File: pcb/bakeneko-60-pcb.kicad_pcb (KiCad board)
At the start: 2 copper layers, 284.7 x 94.2 mm, 154 parts, among them J1 JST SH 4-pin, J2 AVR-ISP-6, SW1 Reset, U1 SRV05-4, U2 ATmega32U4-AU, Y1 16MHz

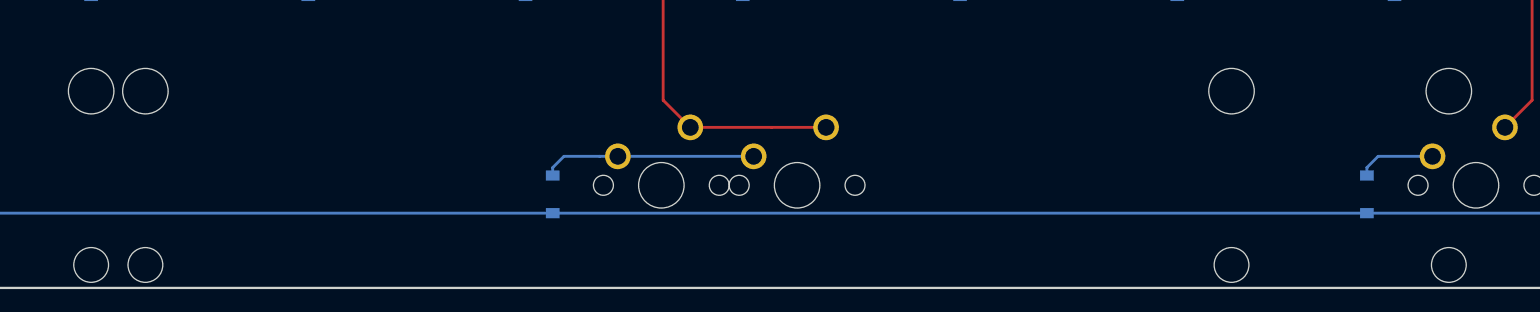
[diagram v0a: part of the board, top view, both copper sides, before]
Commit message: Remove spacebars
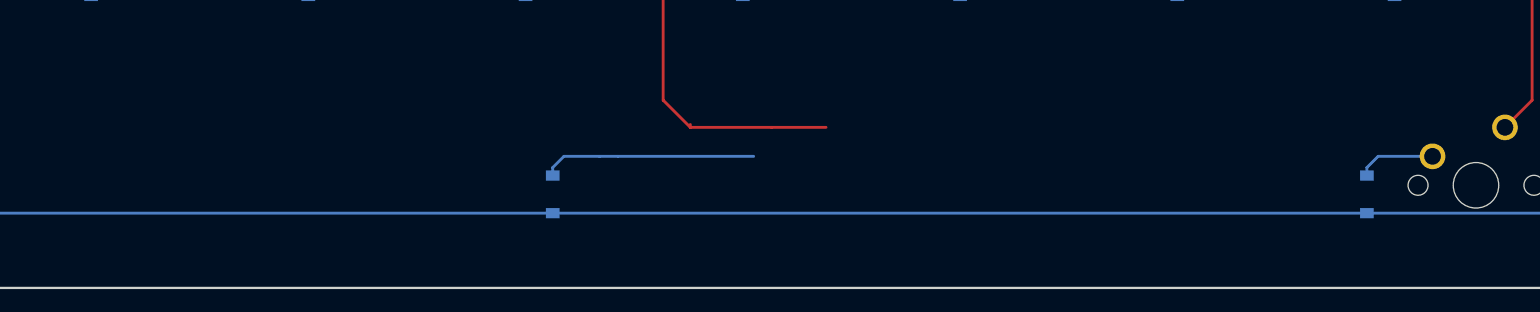
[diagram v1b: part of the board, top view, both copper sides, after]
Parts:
- removed the MX62 at (130.4, 85.2)
- removed MX70: 7u, MX_Only:MXOnly-7U-ReversedStabilizers-NoLED
- renumbered MX63 to MX62, MX64 to MX63, MX65 to MX64, MX66 to MX65, MX67 to MX66, MX68 to MX67, MX69 to MX68, MX72 to MX71, MX73 to MX72
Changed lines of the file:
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@@
     (at 201.88125 85.2)
     (attr through_hole)
-    (fp_text reference "MX63" (at 0 3.175) (layer "Dwgs.User")
+    (fp_text reference "MX62" (at 0 3.175) (layer "Dwgs.User")
       (effects (font (size 1 1) (thickness 0.15)))
     )
@@
     (at 225.69375 85.2)
     (attr through_hole)
-    (fp_text reference "MX64" (at 0 3.175) (layer "Dwgs.User")
+    (fp_text reference "MX63" (at 0 3.175) (layer "Dwgs.User")
       (effects (font (size 1 1) (thickness 0.15)))
     )
@@
     (at 249.50625 85.2)
     (attr through_hole)
-    (fp_text reference "MX65" (at 0 3.175) (layer "Dwgs.User")
+    (fp_text reference "MX64" (at 0 3.175) (layer "Dwgs.User")
       (effects (font (size 1 1) (thickness 0.15)))
     )
@@
     (at 273.31875 85.2)
     (attr through_hole)
-    (fp_text reference "MX66" (at 0 3.175) (layer "Dwgs.User")
+    (fp_text reference "MX65" (at 0 3.175) (layer "Dwgs.User")
       (effects (font (size 1 1) (thickness 0.15)))
     )
@@
     (at 37.575 85.2)
     (attr through_hole)
-    (fp_text reference "MX68" (at 0 3.175) (layer "Dwgs.User")
+    (fp_text reference "MX67" (at 0 3.175) (layer "Dwgs.User")
       (effects (font (size 1 1) (thickness 0.15)))
     )
@@
     (at 61.3875 85.2)
     (attr through_hole)
-    (fp_text reference "MX69" (at 0 3.175) (layer "Dwgs.User")
+    (fp_text reference "MX68" (at 0 3.175) (layer "Dwgs.User")
       (effects (font (size 1 1) (thickness 0.15)))
     )
@@
       (net 80 "COL2"))
   )
-  (footprint "MX_Only:MXOnly-7U-ReversedStabilizers-NoLED" (layer "F.Cu")
-    (at 142.35 85.2)
-    (attr through_hole)
-    (fp_text reference "MX70" (at 0 3.175) (layer "Dwgs.User")
-      (effects (font (size 1 1) (thickness 0.15)))
-    )
-    (fp_text value "7u" (at 0 -7.9375) (layer "Dwgs.User")
-      (effects (font (size 1 1) (thickness 0.15)))
-    )
-    (fp_line (start -7 7) (end -5 7) (layer "Dwgs.User") (width 0.15))
-    (fp_line (start -5 -7) (end -7 -7) (layer "Dwgs.User") (width 0.15))
-    (fp_line (start 5 -7) (end 7 -7) (layer "Dwgs.User") (width 0.15))
-    (fp_line (start -7 5) (end -7 7) (layer "Dwgs.User") (width 0.15))
-    (fp_line (start 7 -7) (end 7 -5) (layer "Dwgs.User") (width 0.15))
-    (fp_line (start 5 7) (end 7 7) (layer "Dwgs.User") (width 0.15))
-    (fp_line (start -7 -7) (end -7 -5) (layer "Dwgs.User") (width 0.15))
-    (fp_line (start 7 7) (end 7 5) (layer "Dwgs.User") (width 0.15))
-    (fp_line (start -66.675 -9.525) (end 66.675 -9.525) (layer "Dwgs.User") (width 0.15))
-    (fp_line (start 66.675 -9.525) (end 66.675 9.525) (layer "Dwgs.User") (width 0.15))
-    (fp_line (start -66.675 9.525) (end -66.675 -9.525) (layer "Dwgs.User") (width 0.15))
-    (fp_line (start -66.675 9.525) (end 66.675 9.525) (layer "Dwgs.User") (width 0.15))
-    (pad "" np_thru_hole circle locked (at -57.15 -8.255) (size 3.9878 3.9878) (drill 3.9878) (layers *.Cu *.Mask))
-    (pad "" np_thru_hole circle locked (at 0 0) (size 3.9878 3.9878) (drill 3.9878) (layers *.Cu *.Mask))
-    (pad "" np_thru_hole circle locked (at 57.15 -8.255) (size 3.9878 3.9878) (drill 3.9878) (layers *.Cu *.Mask))
-    (pad "" np_thru_hole circle locked (at -57.15 6.985) (size 3.048 3.048) (drill 3.048) (layers *.Cu *.Mask))
-    (pad "" np_thru_hole circle locked (at 5.08 0 48.0996) (size 1.75 1.75) (drill 1.75) (layers *.Cu *.Mask))
-    (pad "" np_thru_hole circle locked (at -5.08 0 48.0996) (size 1.75 1.75) (drill 1.75) (layers *.Cu *.Mask))
-    (pad "" np_thru_hole circle locked (at 57.15 6.985) (size 3.048 3.048) (drill 3.048) (layers *.Cu *.Mask))
-    (pad "1" thru_hole circle locked (at -3.81 -2.54) (size 2.25 2.25) (drill 1.47) (layers *.Cu "B.Mask")
-      (net 66 "Net-(D59-Pad2)"))
-    (pad "2" thru_hole circle locked (at 2.54 -5.08) (size 2.25 2.25) (drill 1.47) (layers *.Cu "B.Mask")
-      (net 84 "COL6"))
-  )
   (footprint "MX_Only:MXOnly-1U-NoLED" (layer "F.Cu")
     (at 247.125 85.2)
     (attr through_hole)
-    (fp_text reference "MX72" (at 0 3.175) (layer "Dwgs.User")
+    (fp_text reference "MX71" (at 0 3.175) (layer "Dwgs.User")
       (effects (font (size 1 1) (thickness 0.15)))
     )
@@
     (at 270.9375 85.2)
     (attr through_hole)
-    (fp_text reference "MX73" (at 0 3.175) (layer "Dwgs.User")
+    (fp_text reference "MX72" (at 0 3.175) (layer "Dwgs.User")
       (effects (font (size 1 1) (thickness 0.15)))
     )
@@
       (net 91 "COL13"))
   )
-  (footprint "MX_Only:MXOnly-6.25U-ReversedStabilizers-NoLED" (layer "F.Cu")
-    (at 130.44375 85.2)
-    (attr through_hole)
-    (fp_text reference "MX62" (at 0 3.175) (layer "Dwgs.User")
-      (effects (font (size 1 1) (thickness 0.15)))
-    )
-    (fp_text value "6.25u" (at 0 -7.9375) (layer "Dwgs.User")
-      (effects (font (size 1 1) (thickness 0.15)))
-    )
-    (fp_line (start 7 7) (end 7 5) (layer "Dwgs.User") (width 0.15))
-    (fp_line (start -59.53125 -9.525) (end 59.53125 -9.525) (layer "Dwgs.User") (width 0.15))
-    (fp_line (start -59.53125 9.525) (end 59.53125 9.525) (layer "Dwgs.User") (width 0.15))
-    (fp_line (start -7 -7) (end -7 -5) (layer "Dwgs.User") (width 0.15))
-    (fp_line (start -59.53125 9.525) (end -59.53125 -9.525) (layer "Dwgs.User") (width 0.15))
-    (fp_line (start -7 5) (end -7 7) (layer "Dwgs.User") (width 0.15))
-    (fp_line (start -7 7) (end -5 7) (layer "Dwgs.User") (width 0.15))
-    (fp_line (start -5 -7) (end -7 -7) (layer "Dwgs.User") (width 0.15))
-    (fp_line (start 7 -7) (end 7 -5) (layer "Dwgs.User") (width 0.15))
-    (fp_line (start 5 7) (end 7 7) (layer "Dwgs.User") (width 0.15))
-    (fp_line (start 59.53125 -9.525) (end 59.53125 9.525) (layer "Dwgs.User") (width 0.15))
-    (fp_line (start 5 -7) (end 7 -7) (layer "Dwgs.User") (width 0.15))
-    (pad "" np_thru_hole circle locked (at 5.08 0 48.0996) (size 1.75 1.75) (drill 1.75) (layers *.Cu *.Mask))
-    (pad "" np_thru_hole circle locked (at -5.08 0 48.0996) (size 1.75 1.75) (drill 1.75) (layers *.Cu *.Mask))
-    (pad "" np_thru_hole circle locked (at -49.9999 6.985) (size 3.048 3.048) (drill 3.048) (layers *.Cu *.Mask))
-    (pad "" np_thru_hole circle locked (at -49.9999 -8.255) (size 3.9878 3.9878) (drill 3.9878) (layers *.Cu *.Mask))
-    (pad "" np_thru_hole circle locked (at 0 0) (size 3.9878 3.9878) (drill 3.9878) (layers *.Cu *.Mask))
-    (pad "" np_thru_hole circle locked (at 49.9999 6.985) (size 3.048 3.048) (drill 3.048) (layers *.Cu *.Mask))
-    (pad "" np_thru_hole circle locked (at 49.9999 -8.255) (size 3.9878 3.9878) (drill 3.9878) (layers *.Cu *.Mask))
-    (pad "1" thru_hole circle locked (at -3.81 -2.54) (size 2.25 2.25) (drill 1.47) (layers *.Cu "B.Mask")
-      (net 66 "Net-(D59-Pad2)"))
-    (pad "2" thru_hole circle locked (at 2.54 -5.08) (size 2.25 2.25) (drill 1.47) (layers *.Cu "B.Mask")
-      (net 84 "COL6"))
-  )
   (footprint "MX_Only:MXOnly-1.25U-NoLED" (layer "F.Cu")
     (at 11.38125 85.2)
@@
     (at 13.7625 85.2)
     (attr through_hole)
-    (fp_text reference "MX67" (at 0 3.175) (layer "Dwgs.User")
-      (effects (font (size 1 1) (thickness 0.15)))
-    )
+    (fp_text reference "MX66" (at 0 3.175) (layer "Dwgs.User")
+      (effects (font (size 1 1) (thickness 0.15)))
+    )
